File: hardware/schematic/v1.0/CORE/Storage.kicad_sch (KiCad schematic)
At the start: 25 parts, among them U1 TXS02612RTWR, U3 SD_Card

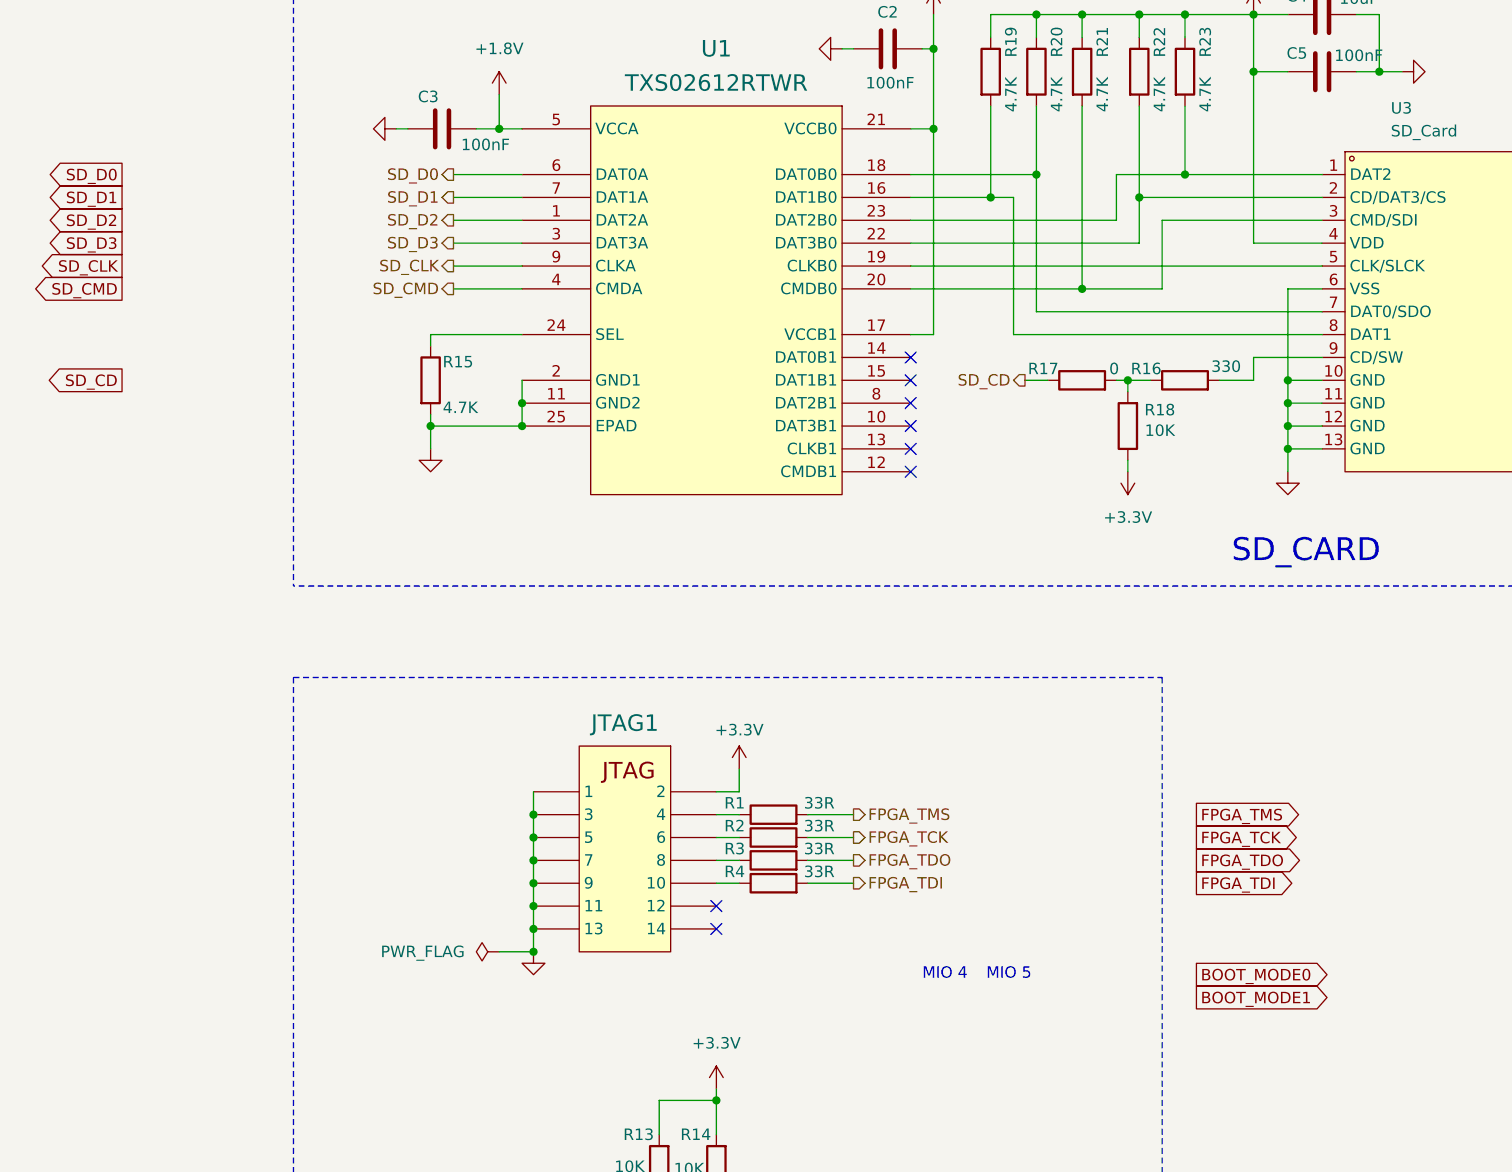
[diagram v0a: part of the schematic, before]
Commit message: sch update
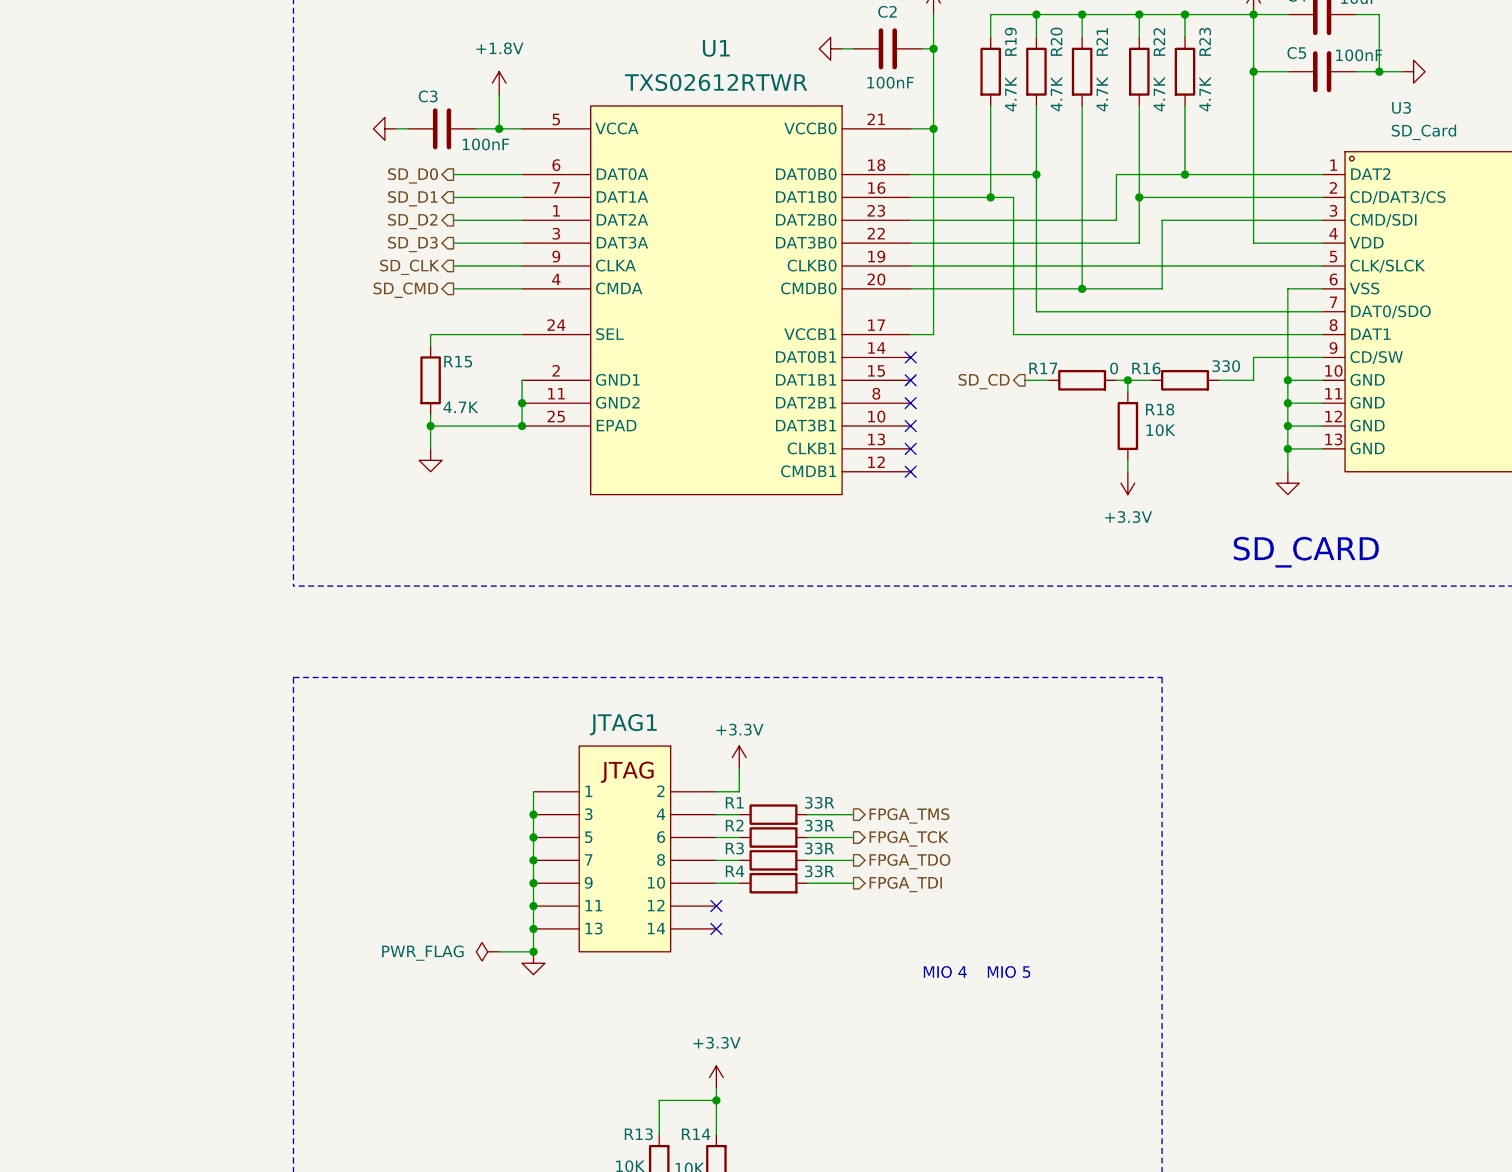
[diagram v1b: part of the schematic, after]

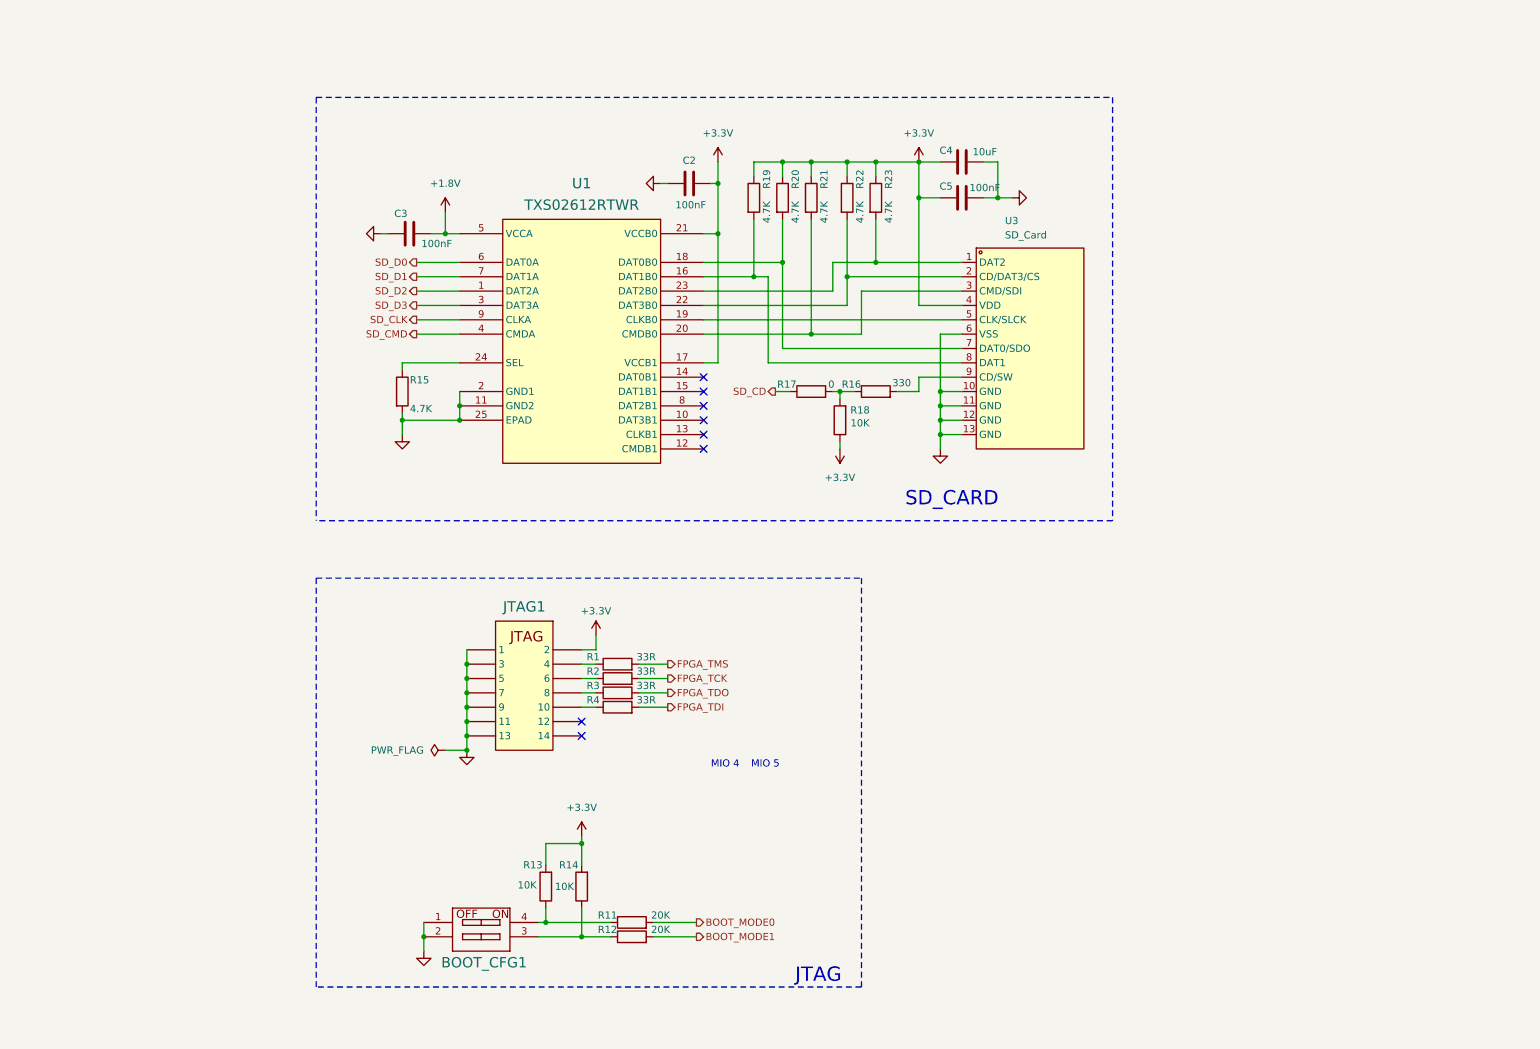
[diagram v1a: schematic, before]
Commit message: sch update
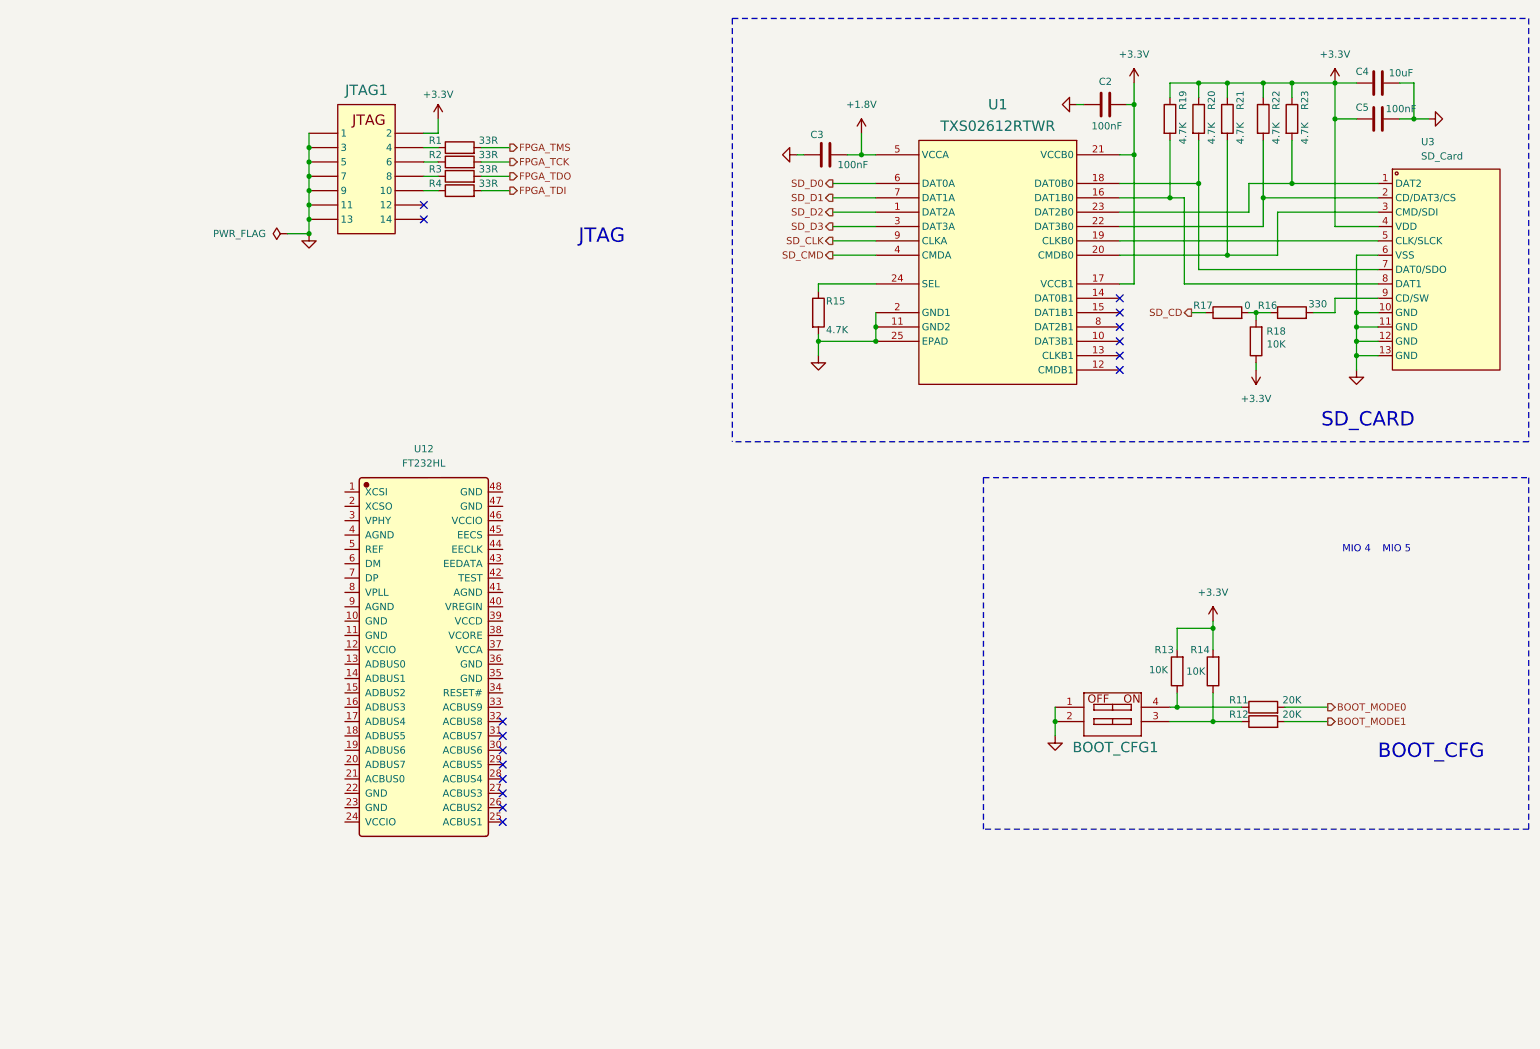
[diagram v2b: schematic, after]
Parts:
- added U12: FT232HL, JLCImport:FT232HL, symbol JLCImport:FT232HL
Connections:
- no-connect marks 8 -> 16
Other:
- note added: "BOOT_CFG"
- moved on the sheet: BOOT_CFG1, C2, C3, C4, C5, JTAG1, R1, R11, R12, R13, R14, R15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

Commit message: sch update
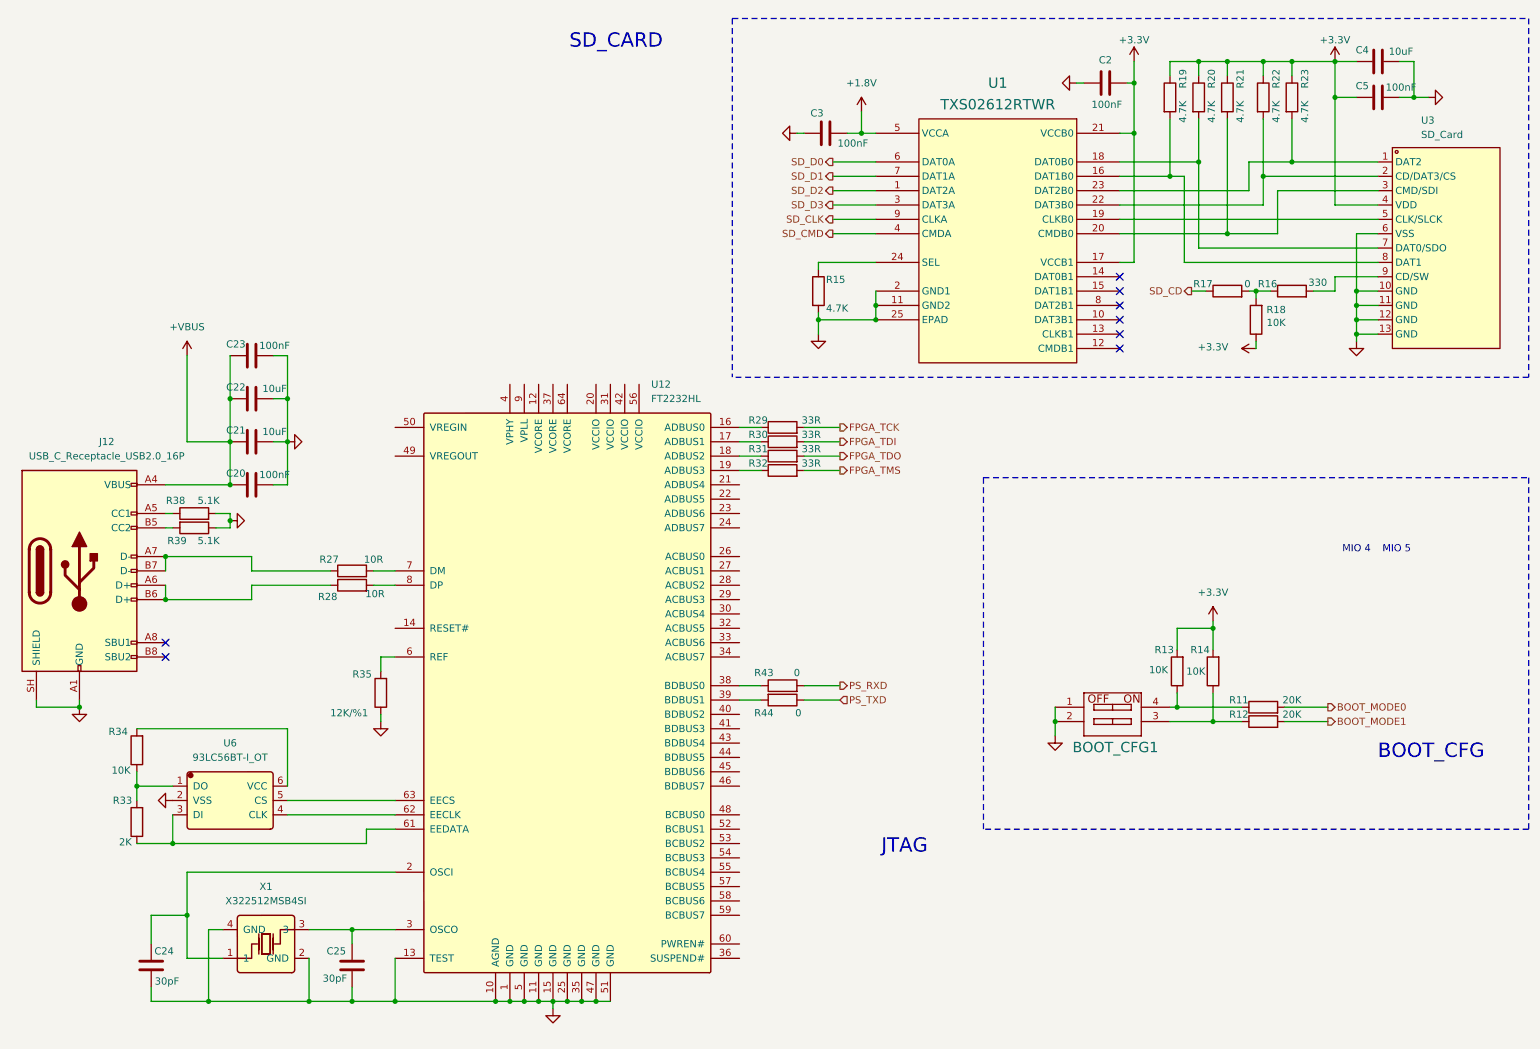
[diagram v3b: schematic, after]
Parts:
- removed JTAG1: JTAG, Counter:DC3_14P_2_7_DIP, symbol Counter:Header 7X2
- removed R1, R2, R3, R4: 33R, Resistor_SMD:R_0402_1005Metric, symbol Device:R
- removed U12: FT232HL, JLCImport:FT232HL, symbol JLCImport:FT232HL
- added C20, C23: 100nF, Capacitor_SMD:C_0402_1005Metric, symbol Device:C
- added C21, C22: 10uF, Capacitor_SMD:C_0603_1608Metric, symbol Device:C
- added C24, C25: 30pF, Capacitor_SMD:C_0402_1005Metric, symbol Device:C
- added J12: USB_C_Receptacle_USB2.0_16P, Connector_USB:USB_C_Receptacle_Palconn_UTC16-G, symbol Connector:USB_C_Receptacle_USB2.0_16P
- added R27, R28: 10R, Resistor_SMD:R_0402_1005Metric, symbol Device:R
- added R29, R30, R31, R32: 33R, Resistor_SMD:R_0402_1005Metric, symbol Device:R
- added R33: 2K, Resistor_SMD:R_0402_1005Metric, symbol Device:R
- added R34: 10K, Resistor_SMD:R_0402_1005Metric, symbol Device:R
- added R35: 12K/%1, Resistor_SMD:R_0402_1005Metric, symbol Device:R
- added R38, R39: 5.1K, Resistor_SMD:R_0402_1005Metric, symbol Device:R
- added R43, R44: 0, Resistor_SMD:R_0402_1005Metric, symbol Device:R
- added U12: FT2232HL, JLCImport:FT2232HL, symbol JLCImport:FT2232HL
- added U6: 93LC56BT-I_OT, JLCImport:93LC56BT-I_OT, symbol JLCImport:93LC56BT-I_OT
- added X1: X322512MSB4SI, JLCImport:X322512MSB4SI, symbol JLCImport:X322512MSB4SI
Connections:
- net FPGA_TCK: now also R29.2
- net FPGA_TDI: now also R30.2
- net FPGA_TDO: now also R31.2
- net FPGA_TMS: now also R32.2
- net GND: now also C20.2, C21.2, C22.2, C23.2, C24.1, C25.1, J12.A1 (GND), J12.A12 (GND), J12.B1 (GND), J12.B12 (GND), J12.SH (SHIELD), R35.1, R38.2, R39.1, U12.1 (GND), U12.10 (AGND), U12.11 (GND), U12.13 (TEST), U12.15 (GND), U12.25 (GND), U12.35 (GND), U12.47 (GND), U12.5 (GND), U12.51 (GND), U6.2 (VSS), X1.2 (GND), X1.4 (GND)
- new net: J12.A6 (D+), J12.B6 (D+), R28.1
- new net: R28.2, U12.8 (DP)
- new net: R32.1, U12.19 (ADBUS3)
- new net: C25.2, U12.3 (OSCO), X1.3
- new net: R31.1, U12.18 (ADBUS2)
- new net: J12.B5 (CC2), R39.2
- new net: R29.1, U12.16 (ADBUS0)
- new net: R30.1, U12.17 (ADBUS1)
- new net: C24.2, U12.2 (OSCI), X1.1
- new net: R43.1, U12.38 (BDBUS0)
- new net: R44.2, U12.39 (BDBUS1)
- new net: R35.2, U12.6 (REF)
- new net: R33.1, U12.61 (EEDATA), U6.3 (DI)
- new net: U12.62 (EECLK), U6.4 (CLK)
- new net: U12.63 (EECS), U6.5 (CS)
- new net: R27.2, U12.7 (DM)
- new net: J12.A7 (D-), J12.B7 (D-), R27.1
- new net: J12.A5 (CC1), R38.1
- new net: R33.2, R34.1, U6.1 (DO)
- new net: R34.2, U6.6 (VCC)
- new net +VBUS: C20.1, C21.1, C22.1, C23.1, J12.A4 (VBUS), J12.A9 (VBUS), J12.B4 (VBUS), J12.B9 (VBUS)
- new net PS_RXD: R43.2
- new net PS_TXD: R44.1
- no-connect marks 16 -> 8
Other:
- moved on the sheet: C2, C3, C4, C5, R15, R16, R17, R18, R19, R20, R21, R22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
